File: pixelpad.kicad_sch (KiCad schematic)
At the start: 4 parts, among them SW1 SW_Push, SW2 SW_Push, SW3 SW_Push, U1 MOUDLE-SEEEDUINO-XIAO

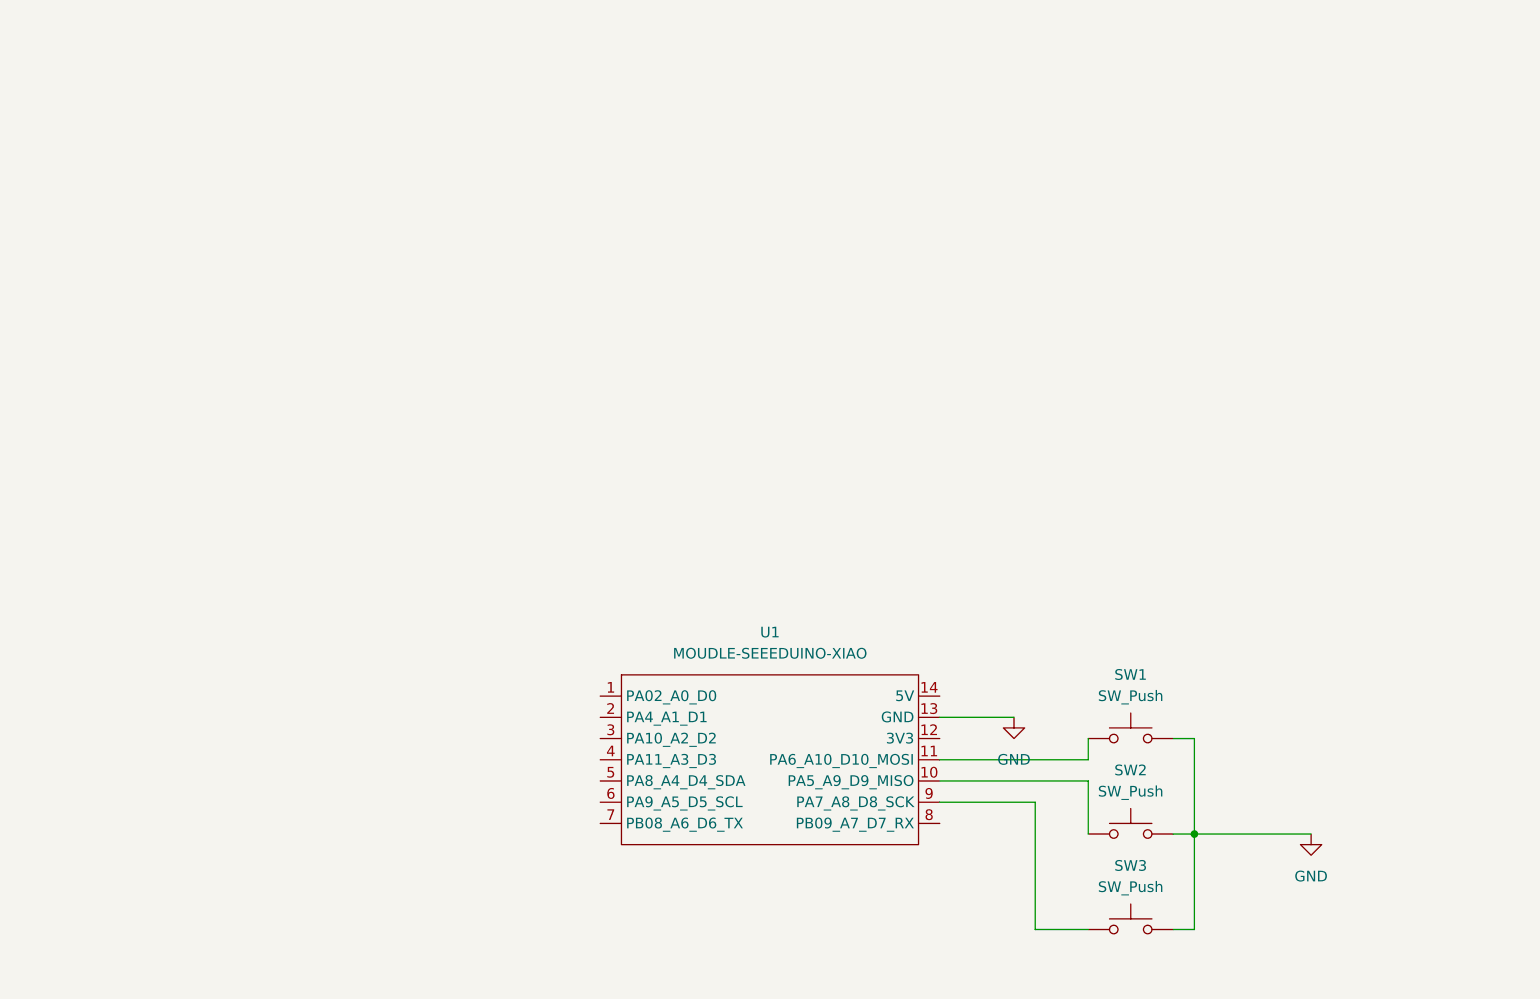
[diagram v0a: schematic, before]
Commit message: I updated the schematic!
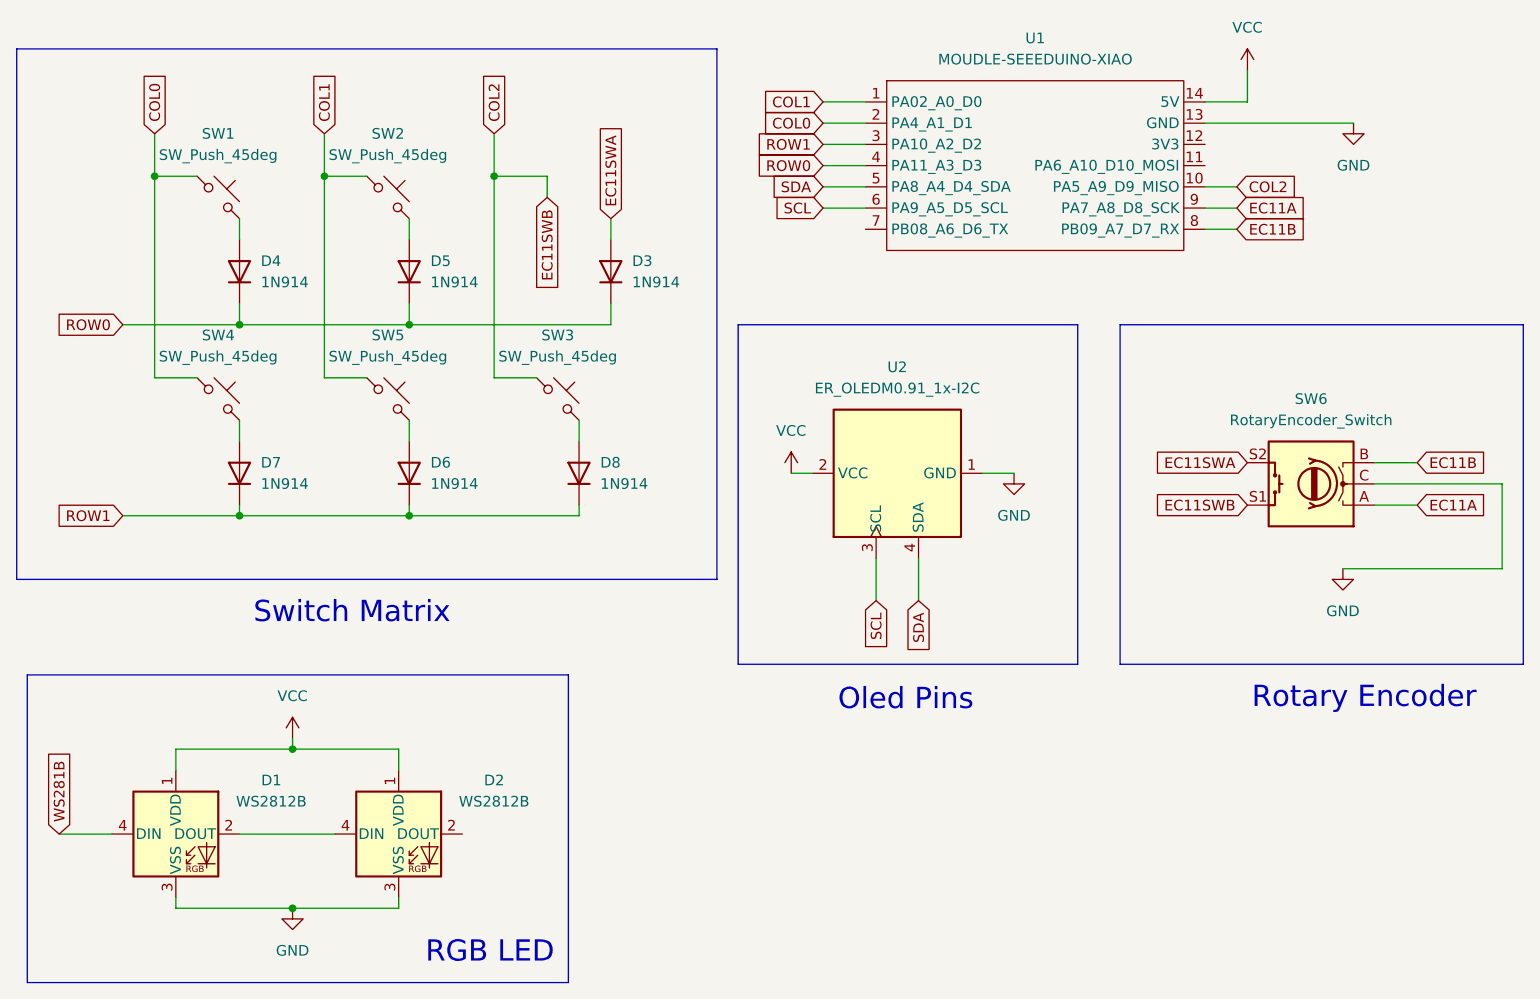
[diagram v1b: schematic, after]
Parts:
- removed SW1, SW2, SW3: SW_Push, Button_Switch_Keyboard:SW_Cherry_MX_1.00u_PCB, symbol KiCad-User:SW_Push
- added D1, D2: WS2812B, LED_SMD:LED_WS2812B_PLCC4_5.0x5.0mm_P3.2mm, symbol KiCad-User:WS2812B
- added D3, D4, D5, D6, D7, D8: 1N914, Diode_THT:D_DO-35_SOD27_P7.62mm_Horizontal, symbol Diode:1N914
- added SW1, SW2, SW3, SW4, SW5: SW_Push_45deg, symbol KiCad-User:SW_Push_45deg
- added SW6: RotaryEncoder_Switch, symbol Device:RotaryEncoder_Switch
- added U2: ER_OLEDM0.91_1x-I2C, Display:ER_OLEDM0.91_1x-I2C, symbol KiCad-User:ER_OLEDM0.91_1x-I2C
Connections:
- net GND: now also D1.3 (VSS), D2.3 (VSS), SW6.C, U2.1 (GND)
- net EC11A: now reaches U1.9 (PA7_A8_D8_SCK)
- net EC11A: now also SW6.A
- net COL2: now reaches U1.10 (PA5_A9_D9_MISO)
- net COL2: now also SW3.1, SW6.S1
- net COL1: now reaches U1.1 (PA02_A0_D0)
- net COL1: now also SW2.1, SW5.1
- net VCC: now reaches U1.14 (5V)
- net VCC: now also D1.1 (VDD), D2.1 (VDD), U2.2 (VCC)
- net COL0: now reaches U1.2 (PA4_A1_D1)
- net COL0: now also SW1.1, SW4.1
- net ROW1: now reaches U1.3 (PA10_A2_D2)
- net ROW1: now also D6.1 (K), D7.1 (K), D8.1 (K)
- net ROW0: now reaches U1.4 (PA11_A3_D3)
- net ROW0: now also D3.1 (K), D4.1 (K), D5.1 (K)
- net SDA: now reaches U1.5 (PA8_A4_D4_SDA)
- net SDA: now also U2.4 (SDA)
- net SCL: now reaches U1.6 (PA9_A5_D5_SCL)
- net SCL: now also U2.3 (SCL)
- net EC11B: now reaches U1.8 (PB09_A7_D7_RX)
- net EC11B: now also SW6.B
- new net: D5.2 (A), SW2.2
- new net: D8.2 (A), SW3.2
- new net: D7.2 (A), SW4.2
- new net: D1.2 (DOUT), D2.4 (DIN)
- new net: D4.2 (A), SW1.2
- new net: D6.2 (A), SW5.2
- new net EC11SWA: D3.2 (A), SW6.S2
- new net WS281B: D1.4 (DIN)
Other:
- note added: "Oled Pins"
- note added: "RGB LED"
- note added: "Rotary Encoder"
- note added: "Switch Matrix"
- moved on the sheet: U1
